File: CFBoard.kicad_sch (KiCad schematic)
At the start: 3 parts, among them U1 STM32 Blue Pill, U2 Wemos D1 Mini, U3 GY-6500

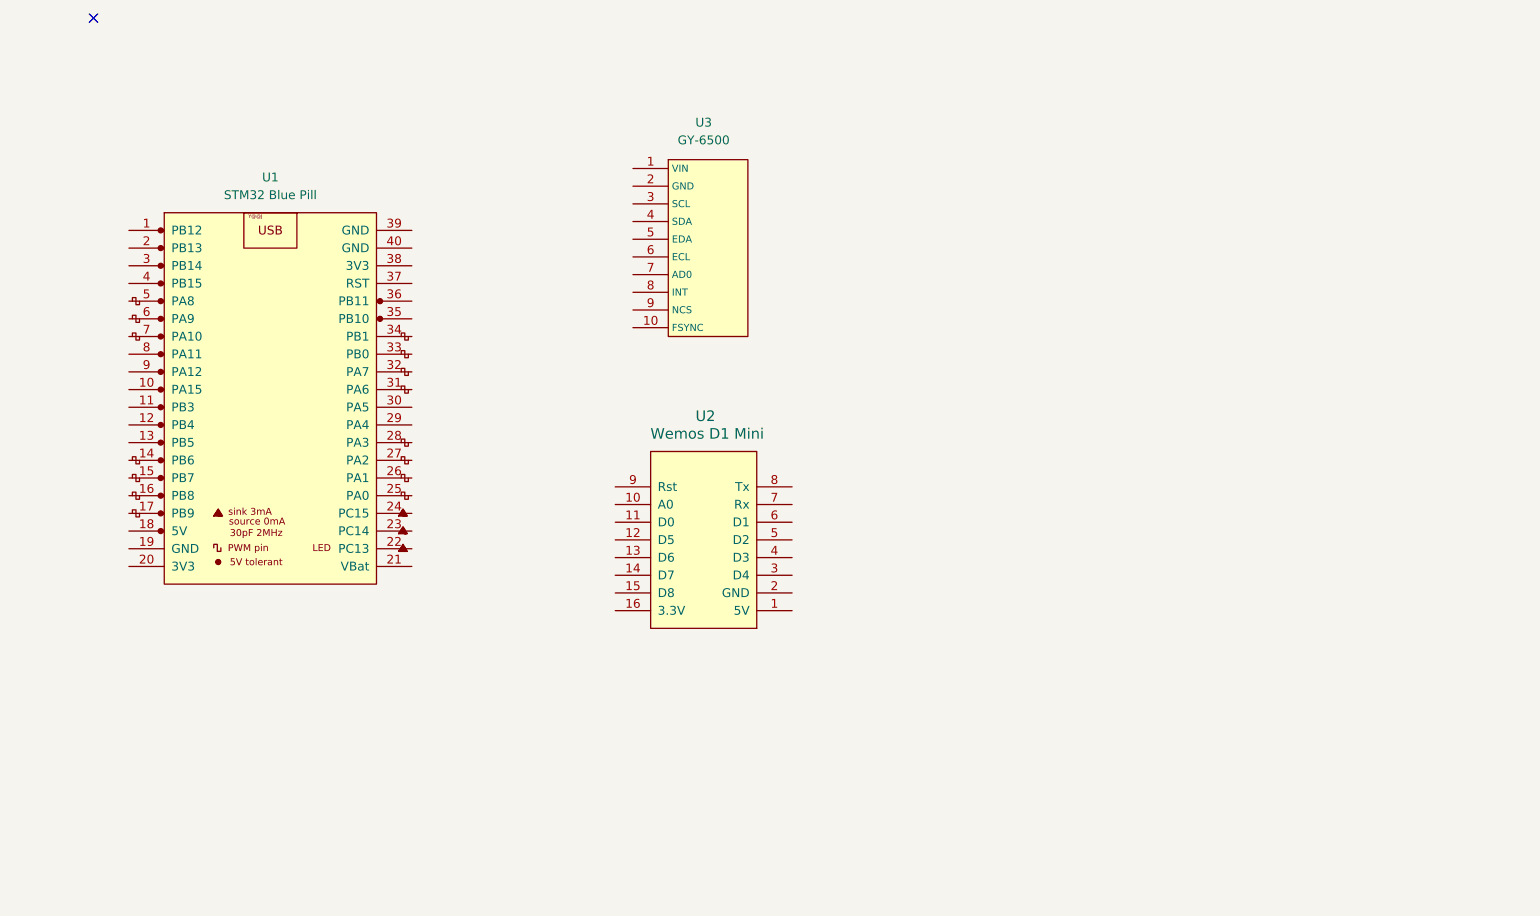
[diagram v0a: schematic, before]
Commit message: feat: layout all the components
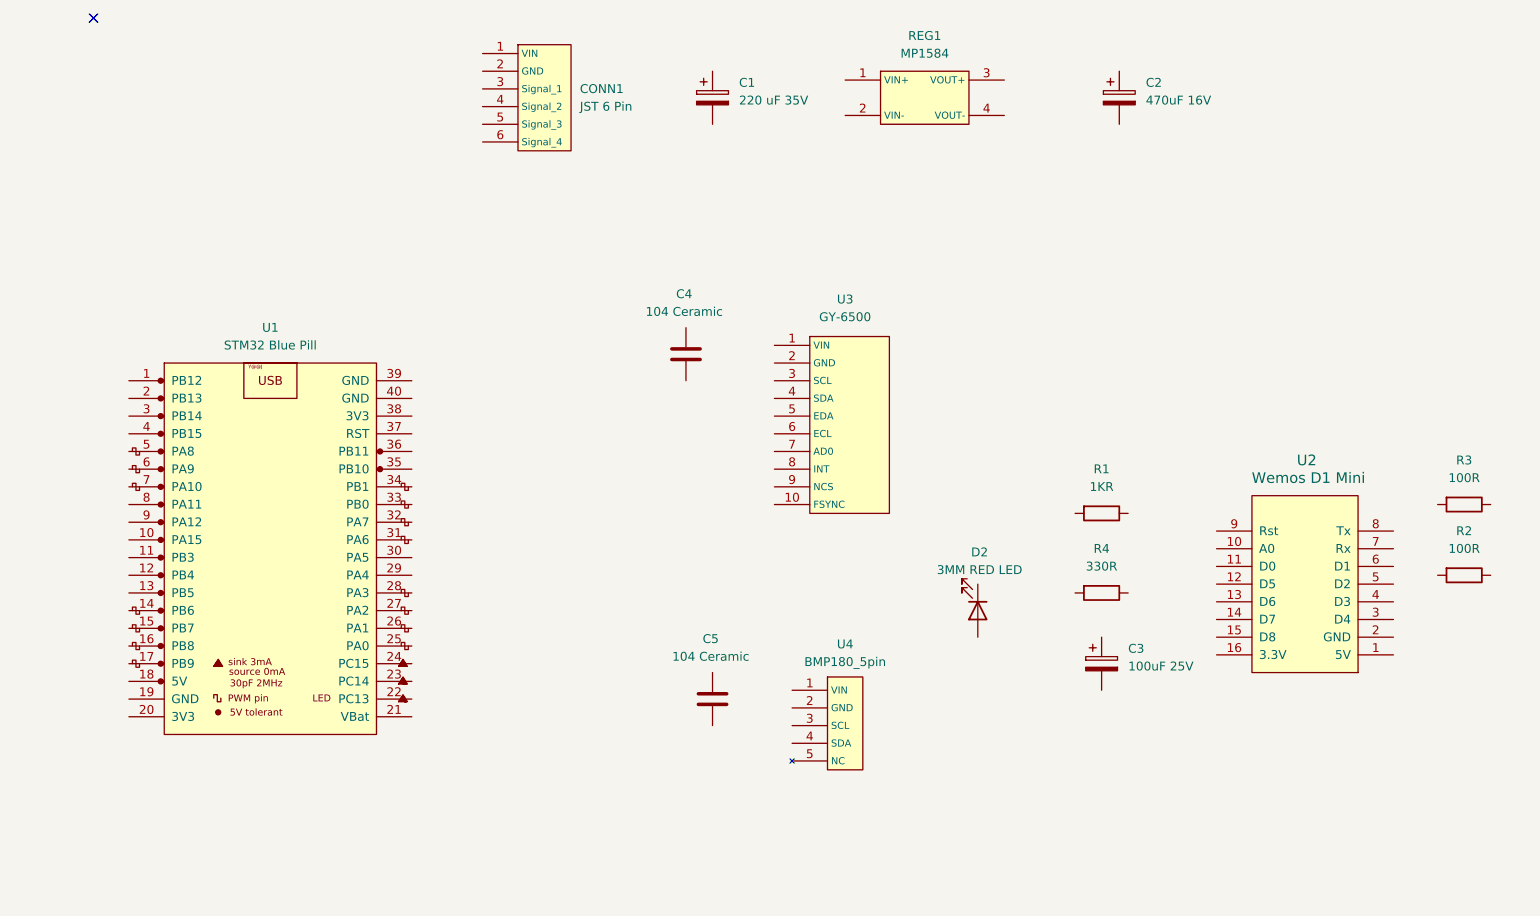
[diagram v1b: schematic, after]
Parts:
- added C1: 220 uF 35V, Capacitor_THT:CP_Radial_D6.3mm_P2.50mm, symbol Device:C_Polarized
- added C2: 470uF 16V, Capacitor_THT:CP_Radial_D5.0mm_P2.50mm, symbol Device:C_Polarized
- added C3: 100uF 25V, Capacitor_THT:CP_Radial_D5.0mm_P2.50mm, symbol Device:C_Polarized
- added C4, C5: 104 Ceramic, Capacitor_THT:C_Disc_D3.0mm_W1.6mm_P2.50mm, symbol Device:C
- added CONN1: JST 6 Pin, Connector_JST:JST_XH_B6B-XH-A_1x06_P2.50mm_Vertical, symbol JST_6pin:JST_XH_6pin
- added D2: 3MM RED LED, LED_THT:LED_D3.0mm, symbol Device:LED
- added R1: 1KR, Resistor_THT:R_Axial_DIN0207_L6.3mm_D2.5mm_P10.16mm_Horizontal, symbol Device:R
- added R2, R3: 100R, Resistor_THT:R_Axial_DIN0207_L6.3mm_D2.5mm_P10.16mm_Horizontal, symbol Device:R
- added R4: 330R, Resistor_THT:R_Axial_DIN0207_L6.3mm_D2.5mm_P10.16mm_Horizontal, symbol Device:R
- added REG1: MP1584, MP1584:MP1584, symbol mp1584:MP1584
- added U4: BMP180_5pin, BMP180:BMP180_5Pin, symbol bmp180:BMP180_5pin
- U1: footprint STM32_Footprints:YAAJ_BluePill_1 -> STM32_Footprints:YAAJ_BluePill_2
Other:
- moved on the sheet: U1, U2, U3

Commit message: feat: pcb layout
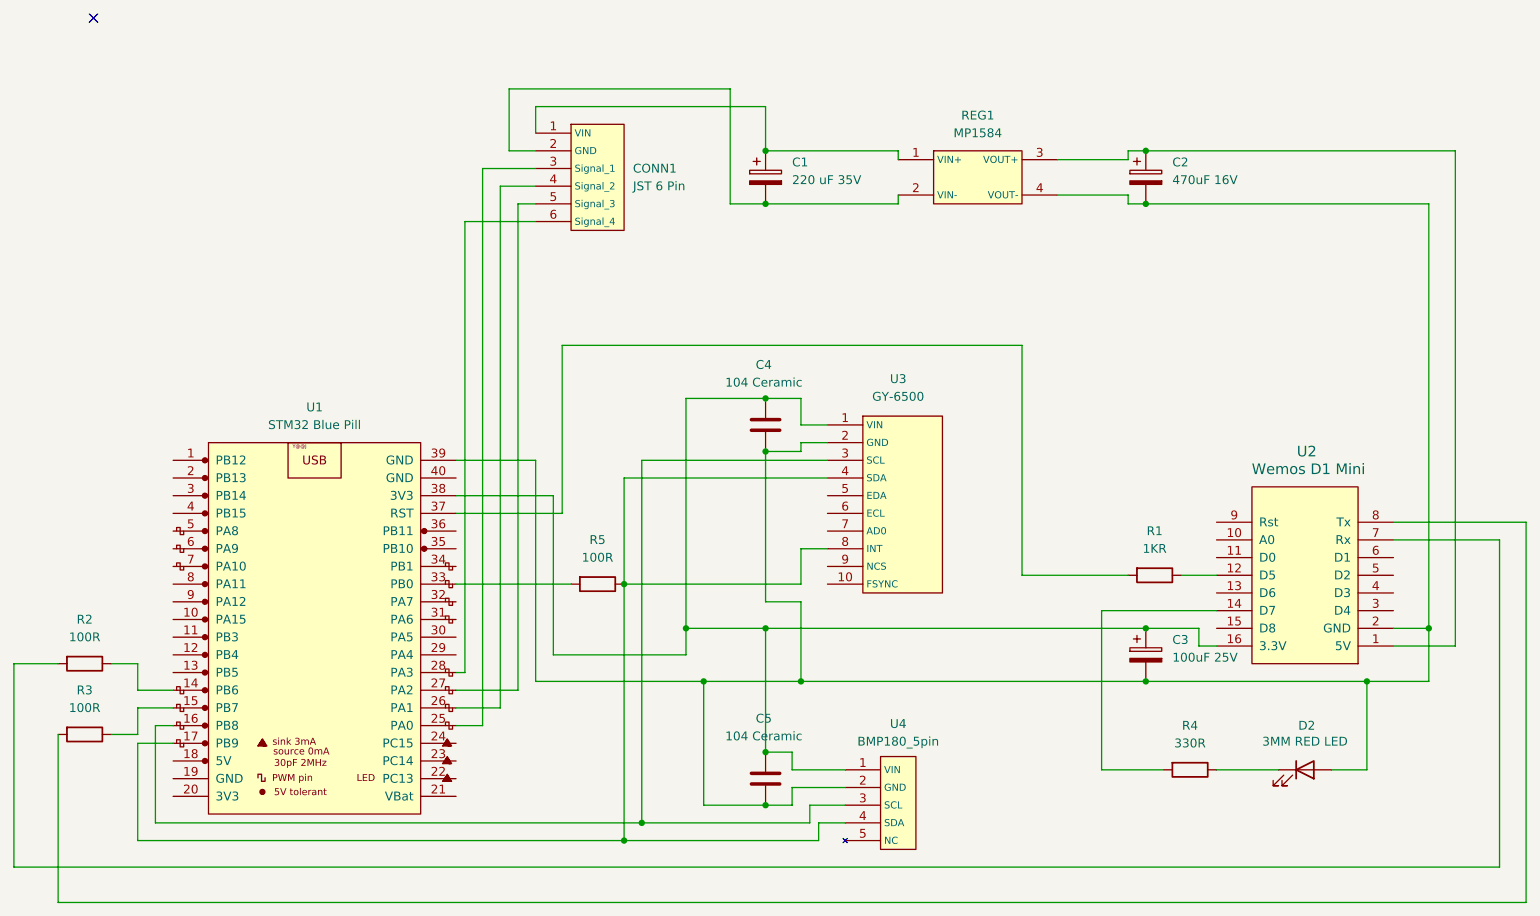
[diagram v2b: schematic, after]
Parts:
- added R5: 100R, R_Axial_DIN0207_L6.3mm_D2.5mm_P7.62mm_Horizontal, symbol Device:R
- R1, R2, R3: footprint Resistor_THT:R_Axial_DIN0207_L6.3mm_D2.5mm_P10.16mm_Horizontal -> R_Axial_DIN0207_L6.3mm_D2.5mm_P7.62mm_Horizontal
- R4: footprint Resistor_THT:R_Axial_DIN0207_L6.3mm_D2.5mm_P10.16mm_Horizontal -> Resistor_THT:R_Axial_DIN0207_L6.3mm_D2.5mm_P7.62mm_Horizontal
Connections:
- net at C3.1: now also C4.1, C5.1, U1.38 (3V3), U2.16 (3.3V), U3.1 (VIN), U4.1 (VIN)
- net at C3.2: now also C2.2, C4.2, C5.2, D2.2 (A), REG1.4 (VOUT-), U1.39 (GND), U2.2 (GND), U3.2 (GND), U4.2 (GND)
- net at R4.1: now also D2.1 (K)
- net at R4.2: now also U2.14 (D7)
- net at U3.3 (SCL): now also U1.16 (PB8), U4.3 (SCL)
- net at U3.4 (SDA): now also U1.17 (PB9), U3.8 (INT), U4.4 (SDA), R5.1
- net at U1.14 (PB6): now also R2.1
- net at U1.15 (PB7): now also R3.1
- net at U1.25 (PA0): now also CONN1.3 (Signal_1)
- net at U1.26 (PA1): now also CONN1.4 (Signal_2)
- net at U1.27 (PA2): now also CONN1.5 (Signal_3)
- net at U1.28 (PA3): now also CONN1.6 (Signal_4)
- net at U1.33 (PB0): now also R5.2
- net at U1.37 (RST): now also R1.2
- net at REG1.1 (VIN+): now also C1.1, CONN1.1 (VIN)
- net at REG1.2 (VIN-): now also C1.2, CONN1.2 (GND)
- net at REG1.3 (VOUT+): now also C2.1, U2.1 (5V)
- net at R3.2: now also U2.8 (Tx)
- net at U2.12 (D5): now also R1.1
- net at U2.7 (Rx): now also R2.2
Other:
- moved on the sheet: C1, C2, C3, C4, C5, CONN1, D2, R1, R2, R3, R4, REG1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
